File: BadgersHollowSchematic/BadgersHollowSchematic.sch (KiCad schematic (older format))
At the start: 5 parts

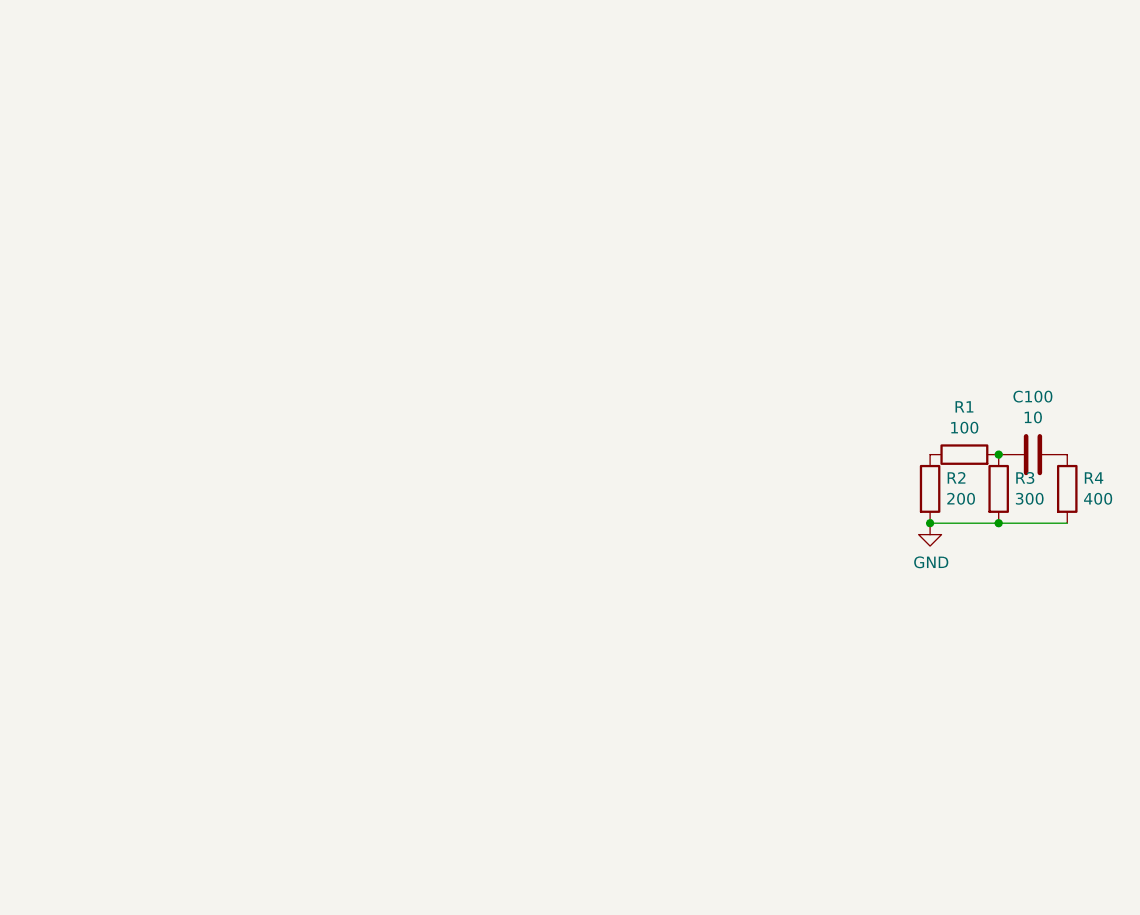
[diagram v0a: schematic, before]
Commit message: Schematic start. mcu and oscillator added
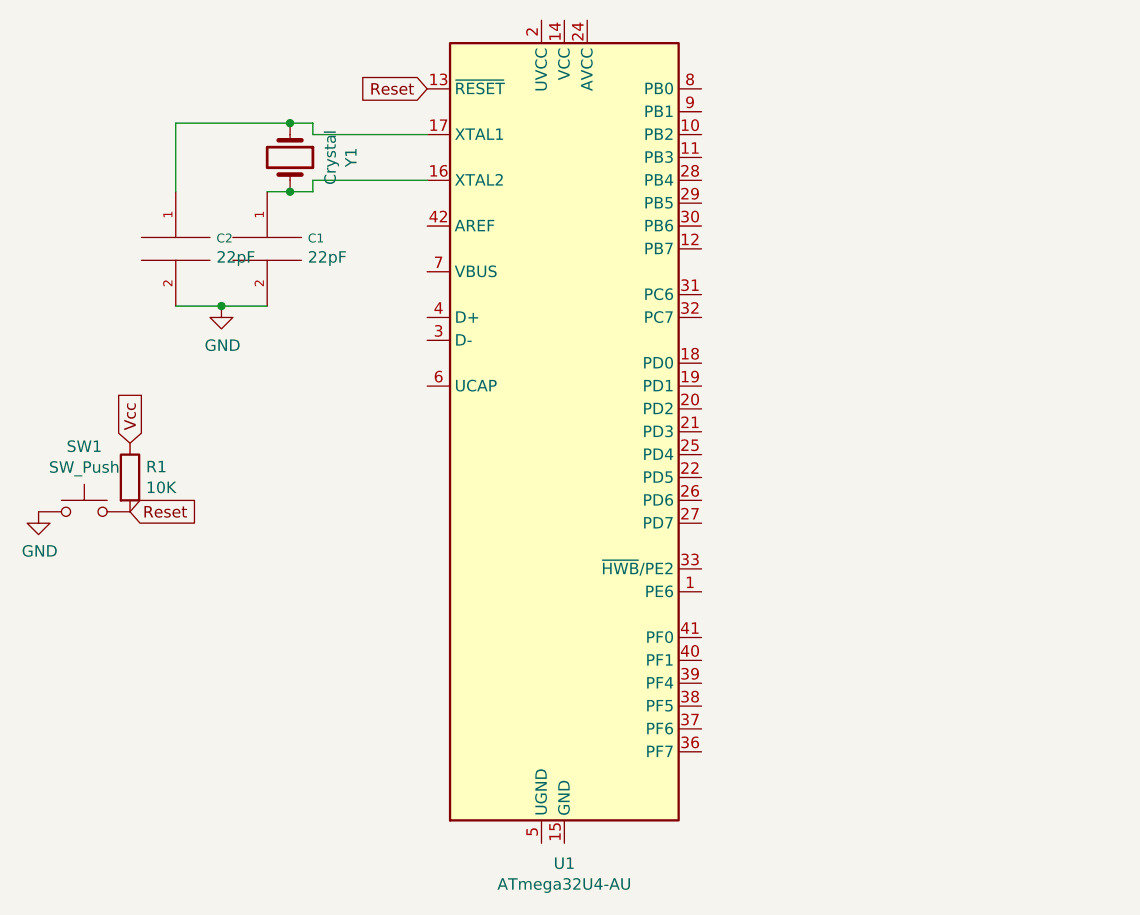
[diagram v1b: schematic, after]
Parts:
- removed C100: 10, Capacitor_THT:CP_Axial_L21.0mm_D8.0mm_P28.00mm_Horizontal, symbol Device:C
- removed R2: 200, Resistor_THT:R_Axial_DIN0204_L3.6mm_D1.6mm_P2.54mm_Vertical, symbol Device:R
- removed R3: 300, Resistor_THT:R_Axial_DIN0207_L6.3mm_D2.5mm_P2.54mm_Vertical, symbol Device:R
- removed R4: 400, Resistor_THT:R_Axial_DIN0204_L3.6mm_D1.6mm_P5.08mm_Vertical, symbol Device:R
- added C1, C2: 22pF, Capacitor_SMD:C_1206_3216Metric_Pad1.42x1.75mm_HandSolder, symbol pspice:C
- added SW1: SW_Push, symbol Switch:SW_Push
- added U1: ATmega32U4-AU, Package_QFP:TQFP-44_10x10mm_P0.8mm, symbol MCU_Microchip_ATmega:ATmega32U4-AU
- added Y1: Crystal, Crystal:Crystal_HC49-U_Vertical, symbol Device:Crystal
- R1: value 100 -> 10K; footprint Capacitor_THT:CP_Axial_L21.0mm_D8.0mm_P28.00mm_Horizontal -> Resistor_SMD:R_1206_3216Metric_Pad1.42x1.75mm_HandSolder
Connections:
- net GND: now also C1.2, C2.2, SW1.1
- net Vcc: now reaches R1.1
- net Reset: now reaches R1.2
- net Reset: now also SW1.2, U1.13 (~RESET)
- new net: U1.14 (VCC), U1.34 (VCC)
- new net: U1.15 (GND), U1.23 (GND), U1.35 (GND), U1.43 (GND)
- new net: C1.1, U1.16 (XTAL2), Y1.2
- new net: C2.1, U1.17 (XTAL1), Y1.1
- new net: U1.24 (AVCC), U1.44 (AVCC)
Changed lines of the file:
@@
 EELAYER 30 0
 EELAYER END
-$Descr A4 11693 8268
+$Descr A1 33110 23386
 encoding utf-8
 Sheet 1 1
@@
 $EndDescr
 $Comp
-L Device:R R2
-U 1 1 5F5AC84A
-P 4500 2950
-F 0 "R2" H 4570 2996 50  0000 L CNN
-F 1 "200" H 4570 2905 50  0000 L CNN
-F 2 "Resistor_THT:R_Axial_DIN0204_L3.6mm_D1.6mm_P2.54mm_Vertical" V 4430 2950 50  0001 C CNN
-F 3 "~" H 4500 2950 50  0001 C CNN
-	1    4500 2950
+L MCU_Microchip_ATmega:ATmega32U4-AU U1
+U 1 1 5F60D4EA
+P 2900 2700
+F 0 "U1" H 2900 811 50  0000 C CNN
+F 1 "ATmega32U4-AU" H 2900 720 50  0000 C CNN
+F 2 "Package_QFP:TQFP-44_10x10mm_P0.8mm" H 2900 2700 50  0001 C CIN
+F 3 "http://ww1.microchip.com/downloads/en/DeviceDoc/Atmel-7766-8-bit-AVR-ATmega16U4-32U4_Datasheet.pdf" H 2900 2700 50  0001 C CNN
+	1    2900 2700
+	1    0    0    -1
+$EndComp
+$Comp
+L Device:Crystal Y1
+U 1 1 5F60FD10
+P 1700 1500
+F 0 "Y1" H 1700 1768 50  0000 C CNN
+F 1 "Crystal" H 1700 1677 50  0000 C CNN
+F 2 "Crystal:Crystal_HC49-U_Vertical" H 1700 1500 50  0001 C CNN
+F 3 "https://www.iqdfrequencyproducts.com/products/pn/LFXTAL027945Bulk.pdf" H 1700 1500 50  0001 C CNN
+	1    1700 1500
+	0    1    1    0
+$EndComp
+Wire Wire Line
+	1800 1400 1800 1350
+Wire Wire Line
+	1800 1350 1700 1350
+Wire Wire Line
+	1800 1600 1800 1650
+Wire Wire Line
+	1800 1650 1700 1650
+Connection ~ 1700 1350
+Wire Wire Line
+	1200 1350 1700 1350
+Wire Wire Line
+	1700 1650 1600 1650
+Connection ~ 1700 1650
+Wire Wire Line
+	1400 2150 1600 2150
+Connection ~ 1400 2150
+Wire Wire Line
+	1200 2150 1400 2150
+$Comp
+L pspice:C C1
+U 1 1 5F693B29
+P 1600 1900
+F 0 "C1" H 1778 1946 39  0000 L CNN
+F 1 "22pF" H 1778 1863 50  0000 L CNN
+F 2 "Capacitor_SMD:C_1206_3216Metric_Pad1.42x1.75mm_HandSolder" H 1600 1900 50  0001 C CNN
+F 3 "https://www.iqdfrequencyproducts.com/products/pn/LFXTAL027945Bulk.pdf" H 1600 1900 50  0001 C CNN
+	1    1600 1900
+	1    0    0    -1
+$EndComp
+$Comp
+L pspice:C C2
+U 1 1 5F67FD87
+P 1200 1900
+F 0 "C2" H 1378 1946 39  0000 L CNN
+F 1 "22pF" H 1378 1863 50  0000 L CNN
+F 2 "Capacitor_SMD:C_1206_3216Metric_Pad1.42x1.75mm_HandSolder" H 1200 1900 50  0001 C CNN
+F 3 "https://www.iqdfrequencyproducts.com/products/pn/LFXTAL027945Bulk.pdf" H 1200 1900 50  0001 C CNN
+	1    1200 1900
+	1    0    0    -1
+$EndComp
+$Comp
+L power:GND #PWR?
+U 1 1 5F67F6EF
+P 1400 2150
+F 0 "#PWR?" H 1400 1900 50  0001 C CNN
+F 1 "GND" H 1405 1977 50  0000 C CNN
+F 2 "" H 1400 2150 50  0001 C CNN
+F 3 "" H 1400 2150 50  0001 C CNN
+	1    1400 2150
+	1    0    0    -1
+$EndComp
+Wire Wire Line
+	1200 1350 1200 1650
+Text GLabel 2300 1200 0    50   Input ~ 0
+Reset
+Wire Wire Line
+	1800 1400 2300 1400
+Wire Wire Line
+	1800 1600 2300 1600
+$Comp
+L Switch:SW_Push SW1
+U 1 1 5F6A57AF
+P 800 3050
+F 0 "SW1" H 800 3335 50  0000 C CNN
+F 1 "SW_Push" H 800 3244 50  0000 C CNN
+F 2 "" H 800 3250 50  0001 C CNN
+F 3 "~" H 800 3250 50  0001 C CNN
+	1    800  3050
 	1    0    0    -1
 $EndComp
 $Comp
 L Device:R R1
-U 1 1 5F5ACEBE
-P 4650 2800
-F 0 "R1" V 4857 2800 50  0000 C CNN
-F 1 "100" V 4766 2800 50  0000 C CNN
-F 2 "Capacitor_THT:CP_Axial_L21.0mm_D8.0mm_P28.00mm_Horizontal" V 4580 2800 50  0001 C CNN
-F 3 "~" H 4650 2800 50  0001 C CNN
-	1    4650 2800
-	0    -1   -1   0
-$EndComp
-$Comp
-L Device:R R3
-U 1 1 5F5ACF00
-P 4800 2950
-F 0 "R3" H 4870 2996 50  0000 L CNN
-F 1 "300" H 4870 2905 50  0000 L CNN
-F 2 "Resistor_THT:R_Axial_DIN0207_L6.3mm_D2.5mm_P2.54mm_Vertical" V 4730 2950 50  0001 C CNN
-F 3 "~" H 4800 2950 50  0001 C CNN
-	1    4800 2950
+U 1 1 5F6A608F
+P 1000 2900
+F 0 "R1" H 1070 2946 50  0000 L CNN
+F 1 "10K" H 1070 2855 50  0000 L CNN
+F 2 "Resistor_SMD:R_1206_3216Metric_Pad1.42x1.75mm_HandSolder" V 930 2900 50  0001 C CNN
+F 3 "https://www.mouser.com/datasheet/2/427/rcse3-1761771.pdf" H 1000 2900 50  0001 C CNN
+	1    1000 2900
 	1    0    0    -1
 $EndComp
+Text GLabel 1000 3050 2    50   Input ~ 0
+Reset
 $Comp
-L Device:C C100
-U 1 1 5F5ADC5F
-P 4950 2800
-F 0 "C100" V 4698 2800 50  0000 C CNN
-F 1 "10" V 4789 2800 50  0000 C CNN
-F 2 "Capacitor_THT:CP_Axial_L21.0mm_D8.0mm_P28.00mm_Horizontal" H 4988 2650 50  0001 C CNN
-F 3 "~" H 4950 2800 50  0001 C CNN
-	1    4950 2800
-	0    1    1    0
-$EndComp
-Connection ~ 4800 2800
-$Comp
-L Device:R R4
-U 1 1 5F5AE074
-P 5100 2950
-F 0 "R4" H 5170 2996 50  0000 L CNN
-F 1 "400" H 5170 2905 50  0000 L CNN
-F 2 "Resistor_THT:R_Axial_DIN0204_L3.6mm_D1.6mm_P5.08mm_Vertical" V 5030 2950 50  0001 C CNN
-F 3 "~" H 5100 2950 50  0001 C CNN
-	1    5100 2950
+L power:GND #PWR?
+U 1 1 5F6A6AAC
+P 600 3050
+F 0 "#PWR?" H 600 2800 50  0001 C CNN
+F 1 "GND" H 605 2877 50  0000 C CNN
+F 2 "" H 600 3050 50  0001 C CNN
+F 3 "" H 600 3050 50  0001 C CNN
+	1    600  3050
 	1    0    0    -1
 $EndComp
-Wire Wire Line
-	5100 3100 4800 3100
-Connection ~ 4800 3100
-Wire Wire Line
-	4800 3100 4500 3100
-$Comp
-L power:GND #PWR0101
-U 1 1 5F5AF0CB
-P 4500 3100
-F 0 "#PWR0101" H 4500 2850 50  0001 C CNN
-F 1 "GND" H 4505 2927 50  0000 C CNN
-F 2 "" H 4500 3100 50  0001 C CNN
-F 3 "" H 4500 3100 50  0001 C CNN
-	1    4500 3100
-	1    0    0    -1
-$EndComp
-Connection ~ 4500 3100
+Text GLabel 1000 2750 1    50   Input ~ 0
+Vcc
 $EndSCHEMATC
